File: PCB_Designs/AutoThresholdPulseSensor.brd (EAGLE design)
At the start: 50.8 x 55.9 mm, 52 parts

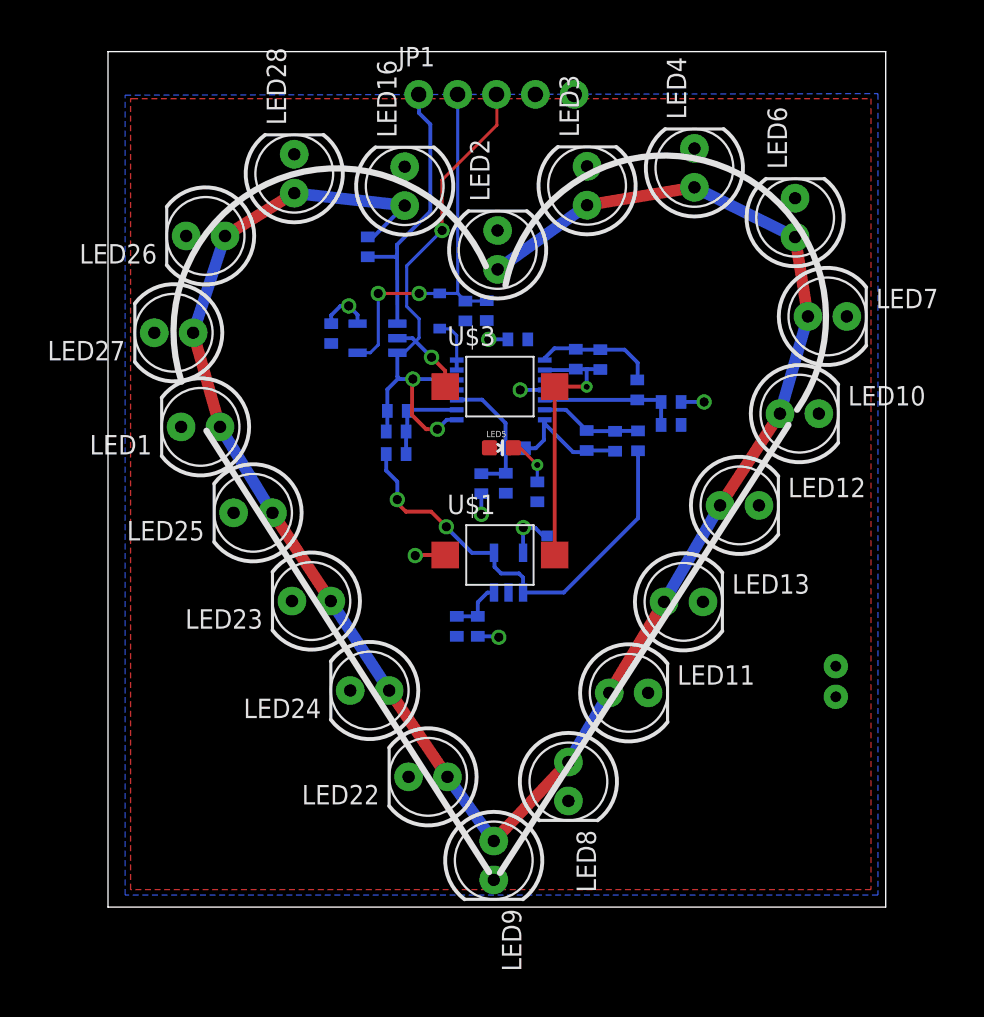
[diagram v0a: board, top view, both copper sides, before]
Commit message: finished first version of board design
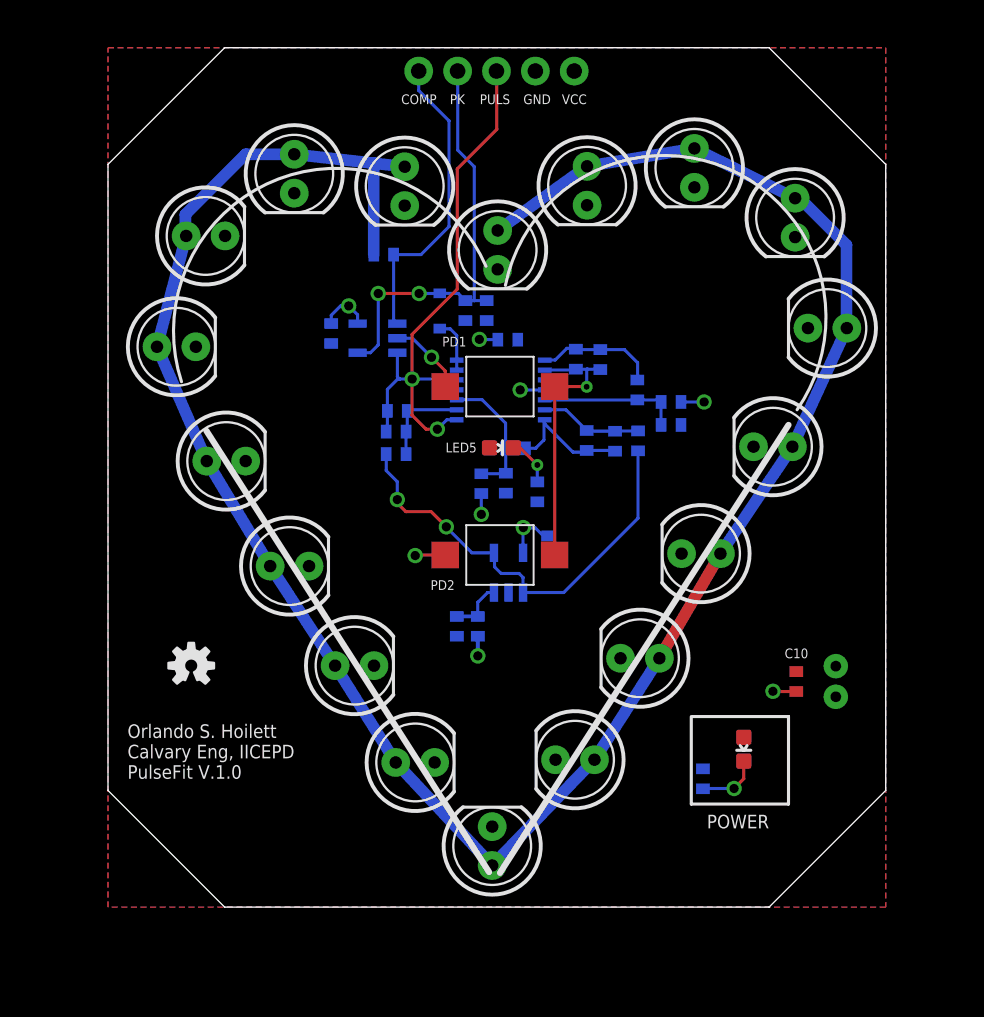
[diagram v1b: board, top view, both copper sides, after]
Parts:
- removed JP1: (no value), SparkFun-Connectors:1X05_NO_SILK
- removed LED13, LED27: (no value), SparkFun-LED:LED5MM
- added BREAKOUT: (no value), SparkFun-Connectors:1X05_NO_SILK
- added C10: 100n, resistor:C0402
- added LOGO1: OSHW-LOGOS, SparkFun-Aesthetics:OSHW-LOGO-S
- added POWER: ON, SparkFun-LED:LED-0603
- added R15: 1k, resistor:R0402
- moved LED1 5.46 mm to (29.9, 36.6), turned to 0 degrees
- moved LED12 4.03 mm to (64.1, 23.1), turned to 180 degrees
- moved LED25 3.81 mm to (33.1, 29.1), turned to 0 degrees
- moved LED10 2.76 mm to (68.8, 30.1), turned to 180 degrees
- moved LED23 2.69 mm to (37.3, 22.3), turned to 0 degrees
- moved LED11 2.38 mm to (60.1, 16.3), turned to 180 degrees
- moved LED24 1.90 mm to (41.5, 15.8), turned to 0 degrees
- moved LED8 1.49 mm to (55.9, 9.63), turned to 180 degrees
- moved LED22 1.26 mm to (45.5, 9.45), turned to 0 degrees
- moved R13 1.16 mm to (43.4, 42.6), turned to 0 degrees
- moved LED9 0.95 mm to (50.5, 3.99), turned to 90 degrees
- moved LED7 0.76 mm to (72.4, 37.8), turned to 180 degrees
- moved C7 0.66 mm to (51.5, 37.1)
- turned LED16 to 270 degrees
- turned LED2 to 270 degrees
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- renumbered U$1 to PD2, U$3 to PD1, U$4 to JST
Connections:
- new net N$12: POWER.C, R15.1
- net ANODE: no longer LED13.A, LED27.A
- net COMP: now also BREAKOUT.1; no longer JP1.1
- net GND: now also BREAKOUT.4, C10.2, R15.2; no longer JP1.4, LED13.K, LED27.K
- net PEAK: now also BREAKOUT.2; no longer JP1.2
- net PULSE: now also BREAKOUT.3; no longer JP1.3
- net VCC: now also BREAKOUT.5, C10.1, POWER.A; no longer JP1.5
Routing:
- net ANODE: track 128.5 -> 145.5 mm
- net N$12: track 0.00 -> 4.09 mm, vias 0 -> 1
- net PEAK: track 25.2 -> 27.7 mm
- net PULSE: track 35.8 -> 38.2 mm, vias 3 -> 2
- net COMP: track 18.1 -> 20.0 mm
- net GND: track 7.01 -> 8.54 mm, vias 2 -> 3
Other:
- board size 50.8 x 55.9 mm -> 50.8 x 56.1 mm
- board text added: "COMP"
- board text added: "GND"
- board text added: "Orlando S. Hoilett Calvary Eng, IICEPD PulseFit V.1.0"
- board text added: "PK"
- board text added: "PULS"
- board text added: "VCC"
